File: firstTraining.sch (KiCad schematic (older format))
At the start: 6 parts

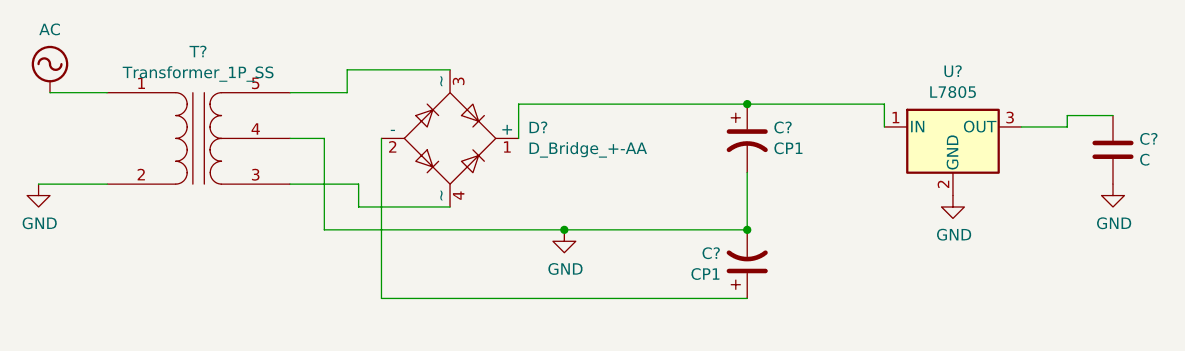
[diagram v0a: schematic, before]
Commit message: 部品の場所を再配置
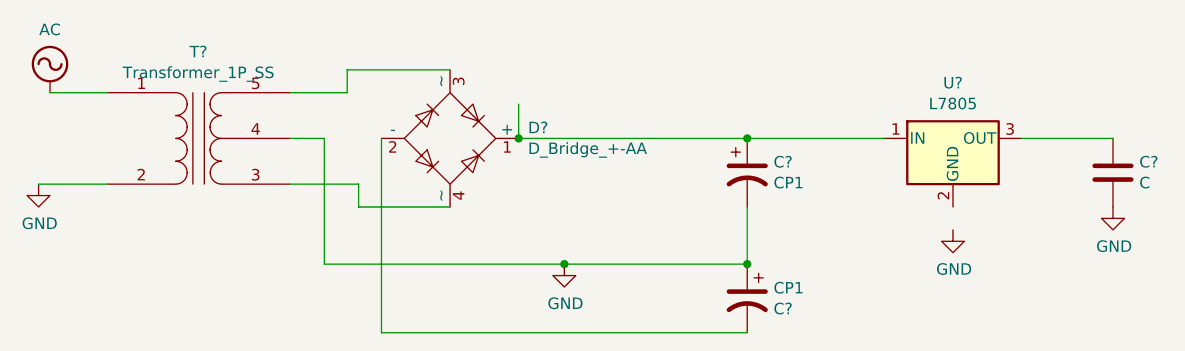
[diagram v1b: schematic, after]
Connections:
- wire segments 22 -> 19
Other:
- moved on the sheet: C?, U?
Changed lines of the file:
@@
 L Device:CP1 C?
 U 1 1 5BD5EB54
-P 4100 1500
-F 0 "C?" H 4215 1546 50  0000 L CNN
-F 1 "CP1" H 4215 1455 50  0000 L CNN
-F 2 "" H 4100 1500 50  0001 C CNN
-F 3 "~" H 4100 1500 50  0001 C CNN
-	1    4100 1500
+P 4100 1650
+F 0 "C?" H 4215 1696 50  0000 L CNN
+F 1 "CP1" H 4215 1605 50  0000 L CNN
+F 2 "" H 4100 1650 50  0001 C CNN
+F 3 "~" H 4100 1650 50  0001 C CNN
+	1    4100 1650
 	1    0    0    -1
 $EndComp
@@
 L Regulator_Linear:L7805 U?
 U 1 1 5BD5FA9A
-P 5000 1450
-F 0 "U?" H 5000 1692 50  0000 C CNN
-F 1 "L7805" H 5000 1601 50  0000 C CNN
-F 2 "" H 5025 1300 50  0001 L CIN
-F 3 "http://www.st.com/content/ccc/resource/technical/document/datasheet/41/4f/b3/b0/12/d4/47/88/CD00000444.pdf/files/CD00000444.pdf/jcr:content/translations/en.CD00000444.pdf" H 5000 1400 50  0001 C CNN
-	1    5000 1450
+P 5000 1500
+F 0 "U?" H 5000 1742 50  0000 C CNN
+F 1 "L7805" H 5000 1651 50  0000 C CNN
+F 2 "" H 5025 1350 50  0001 L CIN
+F 3 "http://www.st.com/content/ccc/resource/technical/document/datasheet/41/4f/b3/b0/12/d4/47/88/CD00000444.pdf/files/CD00000444.pdf/jcr:content/translations/en.CD00000444.pdf" H 5000 1450 50  0001 C CNN
+	1    5000 1500
 	1    0    0    -1
 $EndComp
@@
 L Device:C C?
 U 1 1 5BD5FBB0
-P 5700 1550
-F 0 "C?" H 5815 1596 50  0000 L CNN
-F 1 "C" H 5815 1505 50  0000 L CNN
-F 2 "" H 5738 1400 50  0001 C CNN
-F 3 "~" H 5700 1550 50  0001 C CNN
-	1    5700 1550
+P 5700 1650
+F 0 "C?" H 5815 1696 50  0000 L CNN
+F 1 "C" H 5815 1605 50  0000 L CNN
+F 2 "" H 5738 1500 50  0001 C CNN
+F 3 "~" H 5700 1650 50  0001 C CNN
+	1    5700 1650
 	1    0    0    -1
 $EndComp
@@
 	1300 1700 1000 1700
 Wire Wire Line
-	4100 1900 4100 1650
+	4100 2050 4100 1800
 Wire Wire Line
 	3100 1500 3100 1350
 Wire Wire Line
-	3100 1350 4100 1350
+	3100 1500 4100 1500
 Wire Wire Line
 	2100 1500 2250 1500
 Wire Wire Line
-	2250 1500 2250 1900
+	2250 2050 3300 2050
 Wire Wire Line
-	2250 1900 3300 1900
-Wire Wire Line
-	4100 1350 4700 1350
-Wire Wire Line
-	4700 1350 4700 1450
-Connection ~ 4100 1350
-Wire Wire Line
-	5300 1450 5500 1450
-Wire Wire Line
-	5500 1450 5500 1400
-Wire Wire Line
-	5500 1400 5700 1400
+	4100 1500 4700 1500
+Connection ~ 4100 1500
 $Comp
 L power:GND #PWR?
 U 1 1 5BD66352
-P 5000 1750
-F 0 "#PWR?" H 5000 1500 50  0001 C CNN
-F 1 "GND" H 5005 1577 50  0000 C CNN
-F 2 "" H 5000 1750 50  0001 C CNN
-F 3 "" H 5000 1750 50  0001 C CNN
-	1    5000 1750
+P 5000 1900
+F 0 "#PWR?" H 5000 1650 50  0001 C CNN
+F 1 "GND" H 5005 1727 50  0000 C CNN
+F 2 "" H 5000 1900 50  0001 C CNN
+F 3 "" H 5000 1900 50  0001 C CNN
+	1    5000 1900
 	1    0    0    -1
 $EndComp
@@
 L power:GND #PWR?
 U 1 1 5BD6637E
-P 5700 1700
-F 0 "#PWR?" H 5700 1450 50  0001 C CNN
-F 1 "GND" H 5705 1527 50  0000 C CNN
-F 2 "" H 5700 1700 50  0001 C CNN
-F 3 "" H 5700 1700 50  0001 C CNN
-	1    5700 1700
+P 5700 1800
+F 0 "#PWR?" H 5700 1550 50  0001 C CNN
+F 1 "GND" H 5705 1627 50  0000 C CNN
+F 2 "" H 5700 1800 50  0001 C CNN
+F 3 "" H 5700 1800 50  0001 C CNN
+	1    5700 1800
 	1    0    0    -1
 $EndComp
@@
 L power:GND #PWR?
 U 1 1 5BD663AA
-P 3300 1900
-F 0 "#PWR?" H 3300 1650 50  0001 C CNN
-F 1 "GND" H 3305 1727 50  0000 C CNN
-F 2 "" H 3300 1900 50  0001 C CNN
-F 3 "" H 3300 1900 50  0001 C CNN
-	1    3300 1900
+P 3300 2050
+F 0 "#PWR?" H 3300 1800 50  0001 C CNN
+F 1 "GND" H 3305 1877 50  0000 C CNN
+F 2 "" H 3300 2050 50  0001 C CNN
+F 3 "" H 3300 2050 50  0001 C CNN
+	1    3300 2050
 	1    0    0    -1
 $EndComp
-Connection ~ 3300 1900
+Connection ~ 3300 2050
 Wire Wire Line
-	3300 1900 4100 1900
+	3300 2050 4100 2050
 $Comp
 L Device:CP1 C?
 U 1 1 5BD667AC
-P 4100 2050
-F 0 "C?" H 3985 2004 50  0000 R CNN
-F 1 "CP1" H 3985 2095 50  0000 R CNN
-F 2 "" H 4100 2050 50  0001 C CNN
-F 3 "~" H 4100 2050 50  0001 C CNN
-	1    4100 2050
-	1    0    0    1
+P 4100 2200
+F 0 "C?" H 3985 2154 50  0000 R CNN
+F 1 "CP1" H 3985 2245 50  0000 R CNN
+F 2 "" H 4100 2200 50  0001 C CNN
+F 3 "~" H 4100 2200 50  0001 C CNN
+	1    4100 2200
+	-1   0    0    -1
 $EndComp
-Connection ~ 4100 1900
+Connection ~ 4100 2050
 Wire Wire Line
-	2500 1500 2500 2200
+	2500 2350 4100 2350
 Wire Wire Line
-	2500 2200 4100 2200
+	5300 1500 5700 1500
+Connection ~ 3100 1500
+Wire Wire Line
+	2250 1500 2250 2050
+Wire Wire Line
+	2500 1500 2500 2350
 $EndSCHEMATC
